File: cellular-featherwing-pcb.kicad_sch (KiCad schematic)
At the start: 12 parts, among them J1 SIM8060-6-0-14-00-A, J2 TSM-116-01-L-SV, J3 TSM-112-01-L-SV, J4 U.FL-R-SMT(10), J5 U.FL-R-SMT(10), U1 BG96, U2 TPS63020DSJR, U3 TXB0108DQSR, U4 MAX8868EUK30+

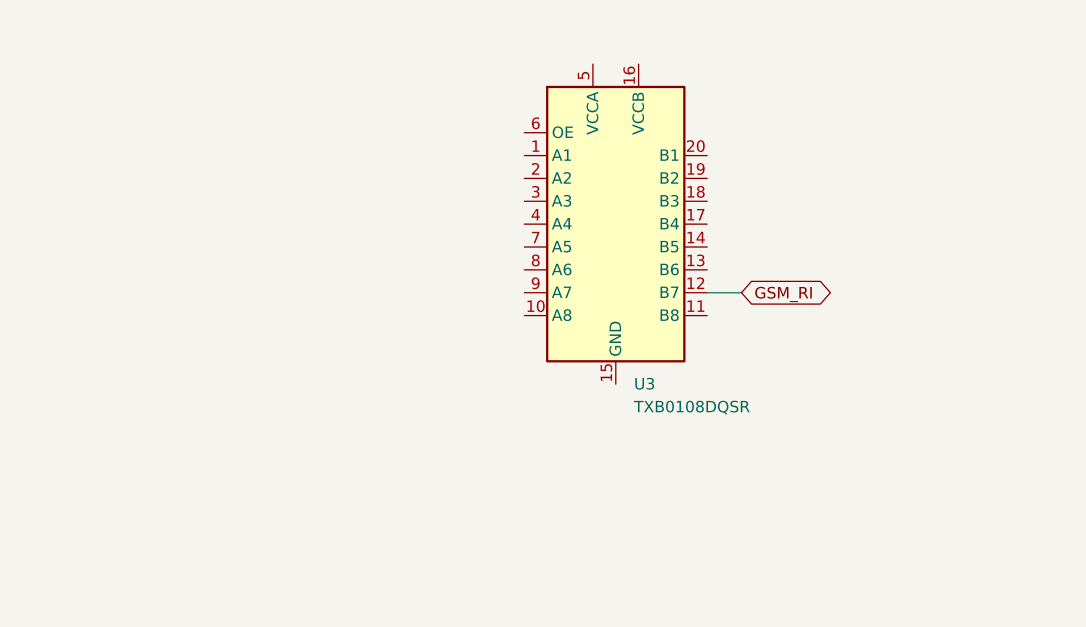
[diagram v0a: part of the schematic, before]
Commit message: schematic updates
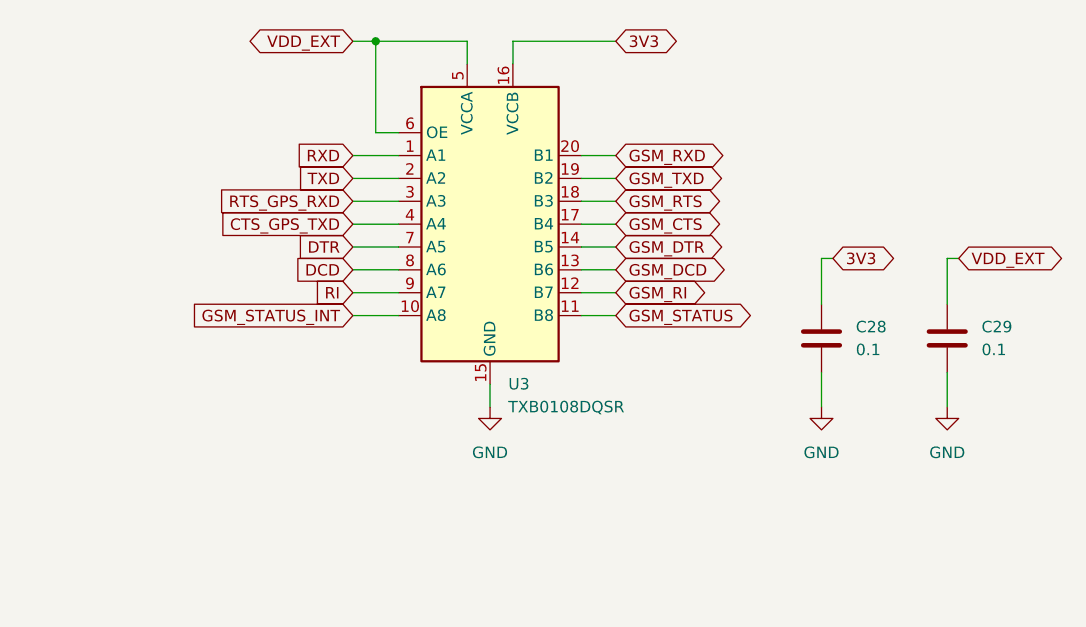
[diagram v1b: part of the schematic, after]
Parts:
- added C28, C29: 0.1, symbol Device:C
- U3: MPN (none) -> TXB0108DQSR
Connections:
- net 3V3: now also U3.16 (VCCB), C28.1
- net DCD: now also U3.8 (A6)
- net DTR: now also U3.7 (A5)
- net GND: now also U3.15 (GND), C28.2, C29.2
- net GSM_STATUS_INT: now also U3.10 (A8)
- net RI: now also U3.9 (A7)
- net RXD: now also U3.1 (A1)
- net TXD: now also U3.2 (A2)
- net VDD_EXT: now also U3.5 (VCCA), U3.6 (OE), C29.1
- net GSM_STATUS: now reaches U3.11 (B8)
- net GSM_DCD: now reaches U3.13 (B6)
- net GSM_DTR: now reaches U3.14 (B5)
- net GSM_CTS: now reaches U3.17 (B4)
- net GSM_RTS: now reaches U3.18 (B3)
- net GSM_TXD: now reaches U3.19 (B2)
- net GSM_RXD: now reaches U3.20 (B1)
- net RTS_GPS_RXD: now reaches U3.3 (A3)
- net CTS_GPS_TXD: now reaches U3.4 (A4)
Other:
- moved on the sheet: U3

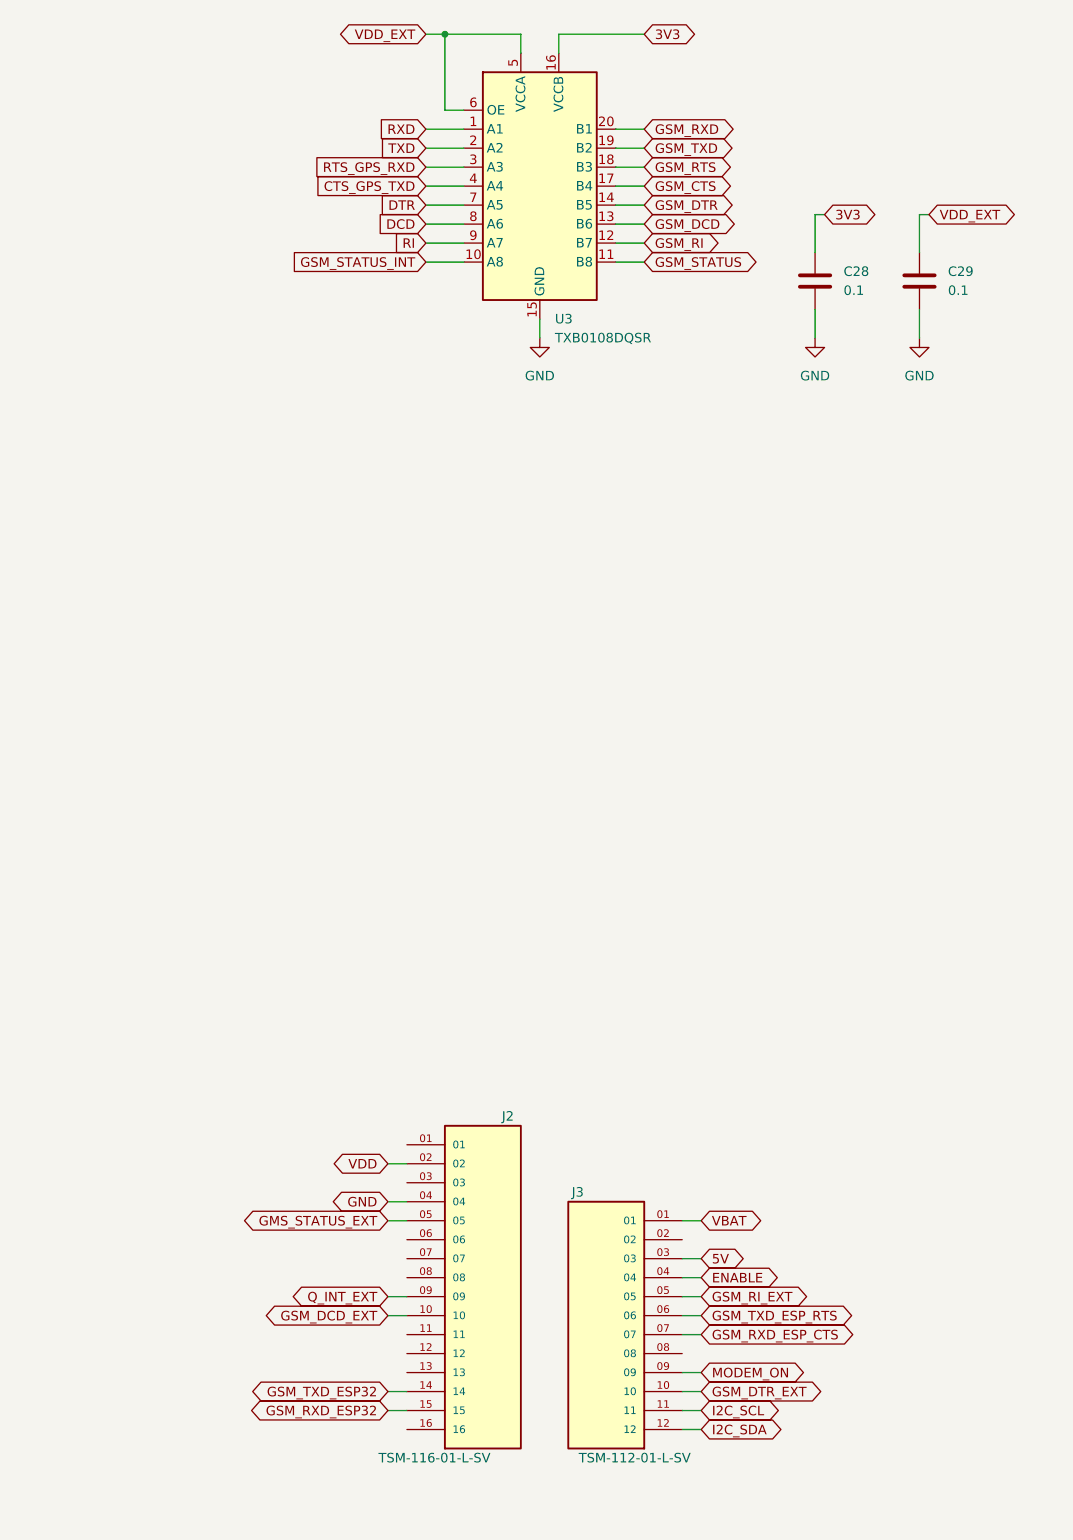
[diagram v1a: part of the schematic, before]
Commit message: More progress
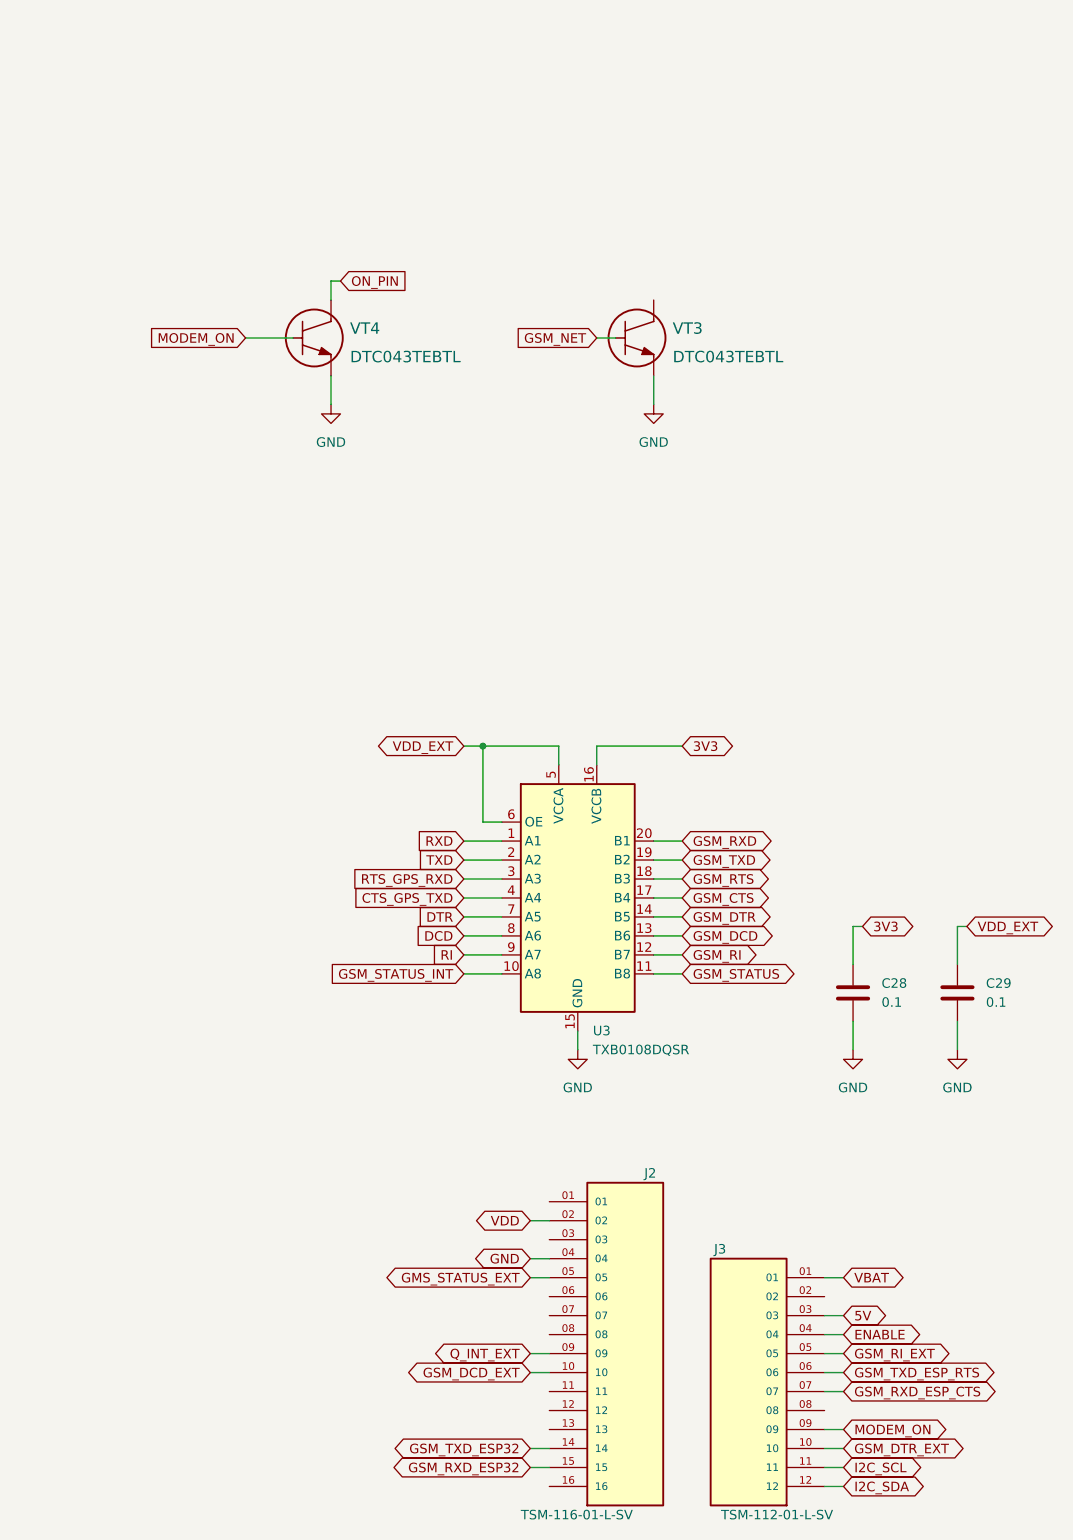
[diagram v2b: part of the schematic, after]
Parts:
- added VT3, VT4: DTC043TEBTL, ul_DTC043TEBTL:DTC043TEBTL, symbol dtc043tebtl:DTC043TEBTL
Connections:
- net GND: now also VT3.3, VT4.3
- net ON_PIN: now also VT4.1, VT4.2
- new net: VT3.1, VT3.2
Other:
- moved on the sheet: C28, C29, J2, J3, U3
